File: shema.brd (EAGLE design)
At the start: 100 x 80 mm, 20 parts

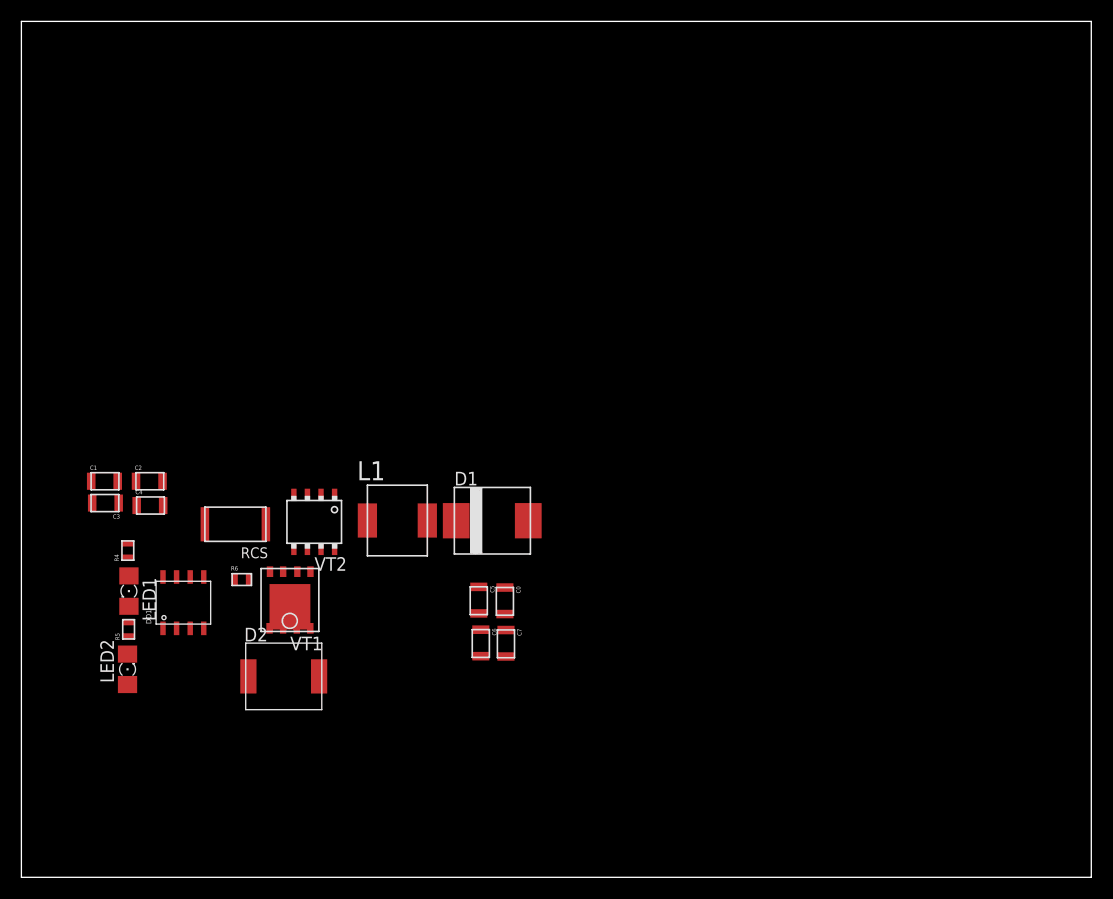
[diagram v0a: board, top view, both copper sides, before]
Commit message: изменения файлов
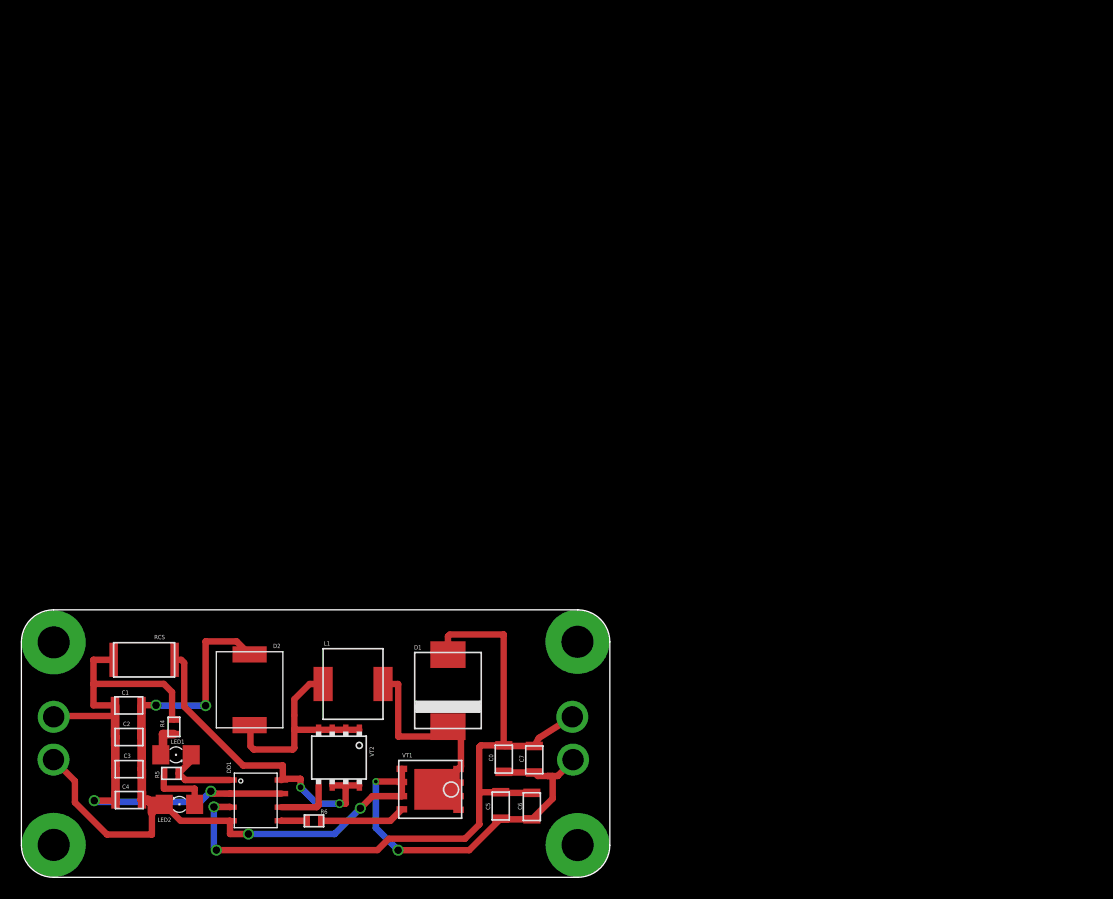
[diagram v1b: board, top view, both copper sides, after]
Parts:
- moved C4 27.6 mm to (10.0, 7.22)
- moved C3 25.0 mm to (10.0, 10.1), turned to 0 degrees
- moved C2 24.0 mm to (10.0, 13.1)
- moved R6 23.5 mm to (27.4, 5.28), turned to 180 degrees
- moved VT2 22.2 mm to (29.7, 11.2)
- moved VT1 22.0 mm to (38.2, 8.22), turned to 270 degrees
- moved C1 21.1 mm to (9.98, 16.1)
- moved DD1 19.7 mm to (21.9, 7.19), turned to 270 degrees
- moved C5 19.3 mm to (44.8, 6.72)
- moved R4 17.0 mm to (14.3, 14.1)
- moved D1 16.4 mm to (39.9, 17.5), turned to 90 degrees
- moved C6 16.0 mm to (47.7, 6.66)
- moved LED1 15.9 mm to (14.4, 11.4), turned to 0 degrees
- moved L1 15.8 mm to (31.0, 18.1)
- moved RCS 15.3 mm to (11.5, 20.3)
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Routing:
- net GND: track 0.00 -> 109.3 mm, vias 0 -> 8
- net 8.4V: track 0.00 -> 70.6 mm, vias 0 -> 3
- net V_IN: track 0.00 -> 54.1 mm, vias 0 -> 3
- net N$4: track 0.00 -> 29.7 mm, vias 0 -> 2
- net N$6: track 0.00 -> 27.1 mm
- net N$5: track 0.00 -> 20.2 mm
- net N$9: track 0.00 -> 7.99 mm
- net N$11: track 0.00 -> 7.29 mm
- net N$1: track 0.00 -> 5.79 mm
- net N$10: track 0.00 -> 5.41 mm
- net N$12: track 0.00 -> 3.05 mm
- net N$8: track 0.00 -> 2.38 mm
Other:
- board size 100 x 80 mm -> 55 x 25 mm
